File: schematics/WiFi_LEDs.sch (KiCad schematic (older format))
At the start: 8 parts

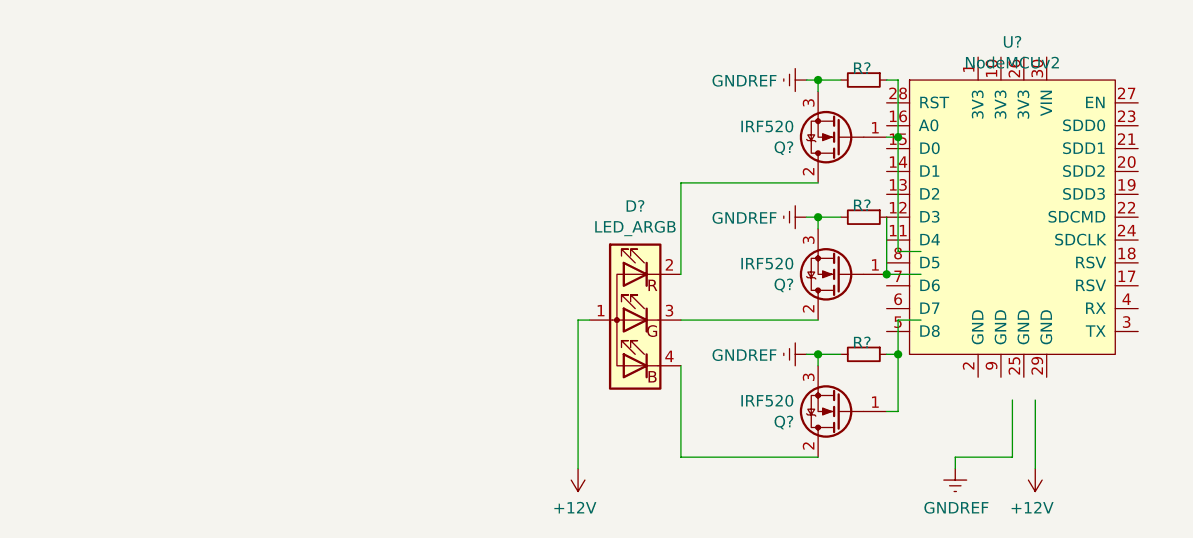
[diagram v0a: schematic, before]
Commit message: Update schematic
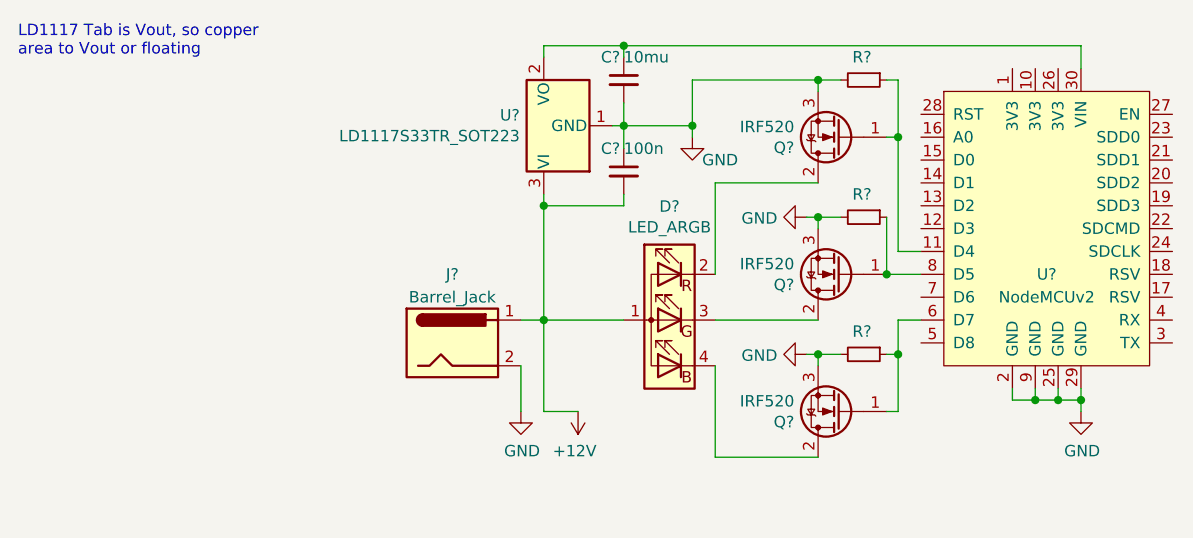
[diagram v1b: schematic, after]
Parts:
- removed U?: NodeMCUv2, symbol WiFi_LEDs:NodeMCUv2
- added C?: 10mu, symbol Device:C_Small
- added C?: 100n, symbol Device:C_Small
- added J?: Barrel_Jack, symbol Connector:Barrel_Jack
- added U?: NodeMCUv2, symbol WiFi_LEDs:NodeMCUv2
- added U?: LD1117S33TR_SOT223, Package_TO_SOT_SMD:SOT-223-3_TabPin2, symbol Regulator_Linear:LD1117S33TR_SOT223
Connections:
- net labels added: GND
- net labels removed: GNDREF
- wire segments 32 -> 54
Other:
- note added: "LD1117 Tab is Vout, so copper\narea to Vout or floating"
- moved on the sheet: D?
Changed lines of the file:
@@
 L power:+12V #PWR?
 U 1 1 60E6F443
-P 3950 3950
-F 0 "#PWR?" H 3950 3800 50  0001 C CNN
-F 1 "+12V" H 3965 4123 50  0000 C CNN
-F 2 "" H 3950 3950 50  0001 C CNN
-F 3 "" H 3950 3950 50  0001 C CNN
-	1    3950 3950
+P 3950 3700
+F 0 "#PWR?" H 3950 3550 50  0001 C CNN
+F 1 "+12V" H 3965 3873 50  0000 C CNN
+F 2 "" H 3950 3700 50  0001 C CNN
+F 3 "" H 3950 3700 50  0001 C CNN
+	1    3950 3700
 	-1   0    0    1
-$EndComp
-$Comp
-L WiFi_LEDs:NodeMCUv2 U?
-U 1 1 60E8A98C
-P 5850 2850
-F 0 "U?" H 5850 3615 50  0000 C CNN
-F 1 "NodeMCUv2" H 5850 3524 50  0000 C CNN
-F 2 "" H 5850 2050 50  0001 C CNN
-F 3 "" H 5850 2050 50  0001 C CNN
-	1    5850 2850
-	1    0    0    -1
-$EndComp
-$Comp
-L power:GNDREF #PWR?
-U 1 1 60F2CBBB
-P 4950 3450
-F 0 "#PWR?" H 4950 3200 50  0001 C CNN
-F 1 "GNDREF" V 4955 3322 50  0000 R CNN
-F 2 "" H 4950 3450 50  0001 C CNN
-F 3 "" H 4950 3450 50  0001 C CNN
-	1    4950 3450
-	0    1    1    0
-$EndComp
-$Comp
-L power:GNDREF #PWR?
-U 1 1 60F2D87A
-P 4950 2850
-F 0 "#PWR?" H 4950 2600 50  0001 C CNN
-F 1 "GNDREF" V 4955 2722 50  0000 R CNN
-F 2 "" H 4950 2850 50  0001 C CNN
-F 3 "" H 4950 2850 50  0001 C CNN
-	1    4950 2850
-	0    1    1    0
-$EndComp
-$Comp
-L power:GNDREF #PWR?
-U 1 1 60F2E231
-P 4950 2250
-F 0 "#PWR?" H 4950 2000 50  0001 C CNN
-F 1 "GNDREF" V 4955 2122 50  0000 R CNN
-F 2 "" H 4950 2250 50  0001 C CNN
-F 3 "" H 4950 2250 50  0001 C CNN
-	1    4950 2250
-	0    1    1    0
 $EndComp
 Wire Wire Line
@@
 $EndComp
 Wire Wire Line
-	4950 2250 5000 2250
-Wire Wire Line
 	5000 2250 5000 2300
 Wire Wire Line
-	3950 3950 3950 3300
-Wire Wire Line
-	3950 3300 4000 3300
-Wire Wire Line
-	4400 3100 4400 2700
-Wire Wire Line
-	4400 3500 4400 3900
-Wire Wire Line
-	4400 3900 5000 3900
-Wire Wire Line
-	4400 3300 5000 3300
+	3800 3300 4150 3300
+Wire Wire Line
+	4550 3100 4550 2700
+Wire Wire Line
+	4550 3500 4550 3900
+Wire Wire Line
+	4550 3900 5000 3900
+Wire Wire Line
+	4550 3300 5000 3300
 $Comp
 L Device:LED_ARGB D?
 U 1 1 61009E65
-P 4200 3300
-F 0 "D?" H 4200 3797 50  0000 C CNN
-F 1 "LED_ARGB" H 4200 3706 50  0000 C CNN
-F 2 "" H 4200 3250 50  0001 C CNN
-F 3 "~" H 4200 3250 50  0001 C CNN
-	1    4200 3300
+P 4350 3300
+F 0 "D?" H 4350 3797 50  0000 C CNN
+F 1 "LED_ARGB" H 4350 3706 50  0000 C CNN
+F 2 "" H 4350 3250 50  0001 C CNN
+F 3 "~" H 4350 3250 50  0001 C CNN
+	1    4350 3300
 	-1   0    0    -1
 $EndComp
 Wire Wire Line
-	4400 2700 5000 2700
+	4550 2700 5000 2700
 Wire Wire Line
 	5300 3100 5450 3100
-$Comp
-L power:+12V #PWR?
-U 1 1 61057791
-P 5950 3950
-F 0 "#PWR?" H 5950 3800 50  0001 C CNN
-F 1 "+12V" H 5965 4123 50  0000 C CNN
-F 2 "" H 5950 3950 50  0001 C CNN
-F 3 "" H 5950 3950 50  0001 C CNN
-	1    5950 3950
-	-1   0    0    1
-$EndComp
-Wire Wire Line
-	5950 3950 5950 3650
-Wire Wire Line
-	5850 3650 5850 3900
-$Comp
-L power:GNDREF #PWR?
-U 1 1 60E6DFF5
-P 5600 3950
-F 0 "#PWR?" H 5600 3700 50  0001 C CNN
-F 1 "GNDREF" H 5605 3777 50  0000 C CNN
-F 2 "" H 5600 3950 50  0001 C CNN
-F 3 "" H 5600 3950 50  0001 C CNN
-	1    5600 3950
-	1    0    0    -1
-$EndComp
-Wire Wire Line
-	5850 3900 5600 3900
-Wire Wire Line
-	5600 3900 5600 3950
 Wire Wire Line
 	5450 3300 5350 3300
@@
 U 1 1 61097AD3
 P 5200 3450
-F 0 "R?" V 5150 3400 50  0000 L CNN
+F 0 "R?" V 5100 3400 50  0000 L CNN
 F 1 "PULLDOWN" V 5150 3200 50  0001 L CNN
 F 2 "" H 5200 3450 50  0001 C CNN
@@
 U 1 1 6109ED31
 P 5200 2850
-F 0 "R?" V 5150 2800 50  0000 L CNN
+F 0 "R?" V 5100 2800 50  0000 L CNN
 F 1 "PULLDOWN" V 5150 2600 50  0001 L CNN
 F 2 "" H 5200 2850 50  0001 C CNN
@@
 U 1 1 610A4161
 P 5200 2250
-F 0 "R?" V 5150 2200 50  0000 L CNN
+F 0 "R?" V 5100 2200 50  0000 L CNN
 F 1 "PULLDOWN" V 5150 2000 50  0001 L CNN
 F 2 "" H 5200 2250 50  0001 C CNN
@@
 Wire Wire Line
 	5100 2250 5000 2250
+Wire Wire Line
+	6150 3600 6150 3650
+$Comp
+L WiFi_LEDs:NodeMCUv2 U?
+U 1 1 60EA9EFB
+P 6000 2900
+F 0 "U?" H 6000 2700 50  0000 C CNN
+F 1 "NodeMCUv2" H 6000 2600 50  0000 C CNN
+F 2 "" H 5850 1950 50  0001 C CNN
+F 3 "" H 5850 1950 50  0001 C CNN
+	1    6000 2900
+	1    0    0    -1
+$EndComp
+$Comp
+L power:GND #PWR?
+U 1 1 60EB2A98
+P 4950 2850
+F 0 "#PWR?" H 4950 2600 50  0001 C CNN
+F 1 "GND" V 4955 2722 50  0000 R CNN
+F 2 "" H 4950 2850 50  0001 C CNN
+F 3 "" H 4950 2850 50  0001 C CNN
+	1    4950 2850
+	0    1    1    0
+$EndComp
+$Comp
+L power:GND #PWR?
+U 1 1 60EB2FC7
+P 4950 3450
+F 0 "#PWR?" H 4950 3200 50  0001 C CNN
+F 1 "GND" V 4955 3322 50  0000 R CNN
+F 2 "" H 4950 3450 50  0001 C CNN
+F 3 "" H 4950 3450 50  0001 C CNN
+	1    4950 3450
+	0    1    1    0
+$EndComp
+$Comp
+L Connector:Barrel_Jack J?
+U 1 1 60EC6BDF
+P 3400 3400
+F 0 "J?" H 3400 3700 50  0000 C CNN
+F 1 "Barrel_Jack" H 3400 3600 50  0000 C CNN
+F 2 "" H 3450 3360 50  0001 C CNN
+F 3 "~" H 3450 3360 50  0001 C CNN
+	1    3400 3400
+	1    0    0    -1
+$EndComp
+Wire Wire Line
+	3700 3300 3800 3300
+$Comp
+L power:GND #PWR?
+U 1 1 60ECA6D3
+P 3700 3700
+F 0 "#PWR?" H 3700 3450 50  0001 C CNN
+F 1 "GND" H 3705 3527 50  0000 C CNN
+F 2 "" H 3700 3700 50  0001 C CNN
+F 3 "" H 3700 3700 50  0001 C CNN
+	1    3700 3700
+	1    0    0    -1
+$EndComp
+Wire Wire Line
+	3700 3500 3700 3700
+Connection ~ 3800 3300
+$Comp
+L Regulator_Linear:LD1117S33TR_SOT223 U?
+U 1 1 60ED508A
+P 3800 2450
+F 0 "U?" V 3846 2555 50  0000 L CNN
+F 1 "LD1117S33TR_SOT223" V 3755 2555 50  0000 L CNN
+F 2 "Package_TO_SOT_SMD:SOT-223-3_TabPin2" H 3800 2650 50  0001 C CNN
+F 3 "http://www.st.com/st-web-ui/static/active/en/resource/technical/document/datasheet/CD00000544.pdf" H 3900 2200 50  0001 C CNN
+	1    3800 2450
+	0    -1   -1   0
+$EndComp
+Wire Wire Line
+	3800 2750 3800 2800
+Wire Wire Line
+	3800 2150 3800 2100
+Wire Wire Line
+	3800 2100 4150 2100
+Wire Wire Line
+	6150 2100 6150 2200
+$Comp
+L power:GND #PWR?
+U 1 1 60EE74C2
+P 4450 2500
+F 0 "#PWR?" H 4450 2250 50  0001 C CNN
+F 1 "GND" H 4650 2400 50  0000 R CNN
+F 2 "" H 4450 2500 50  0001 C CNN
+F 3 "" H 4450 2500 50  0001 C CNN
+	1    4450 2500
+	1    0    0    -1
+$EndComp
+Wire Wire Line
+	5850 3600 5850 3650
+Wire Wire Line
+	5850 3650 5950 3650
+Wire Wire Line
+	5950 3600 5950 3650
+Connection ~ 5950 3650
+Wire Wire Line
+	6050 3600 6050 3650
+Connection ~ 6050 3650
+Wire Wire Line
+	6050 3650 6150 3650
+Wire Wire Line
+	5950 3650 6050 3650
+Connection ~ 6150 3650
+Wire Wire Line
+	6150 3650 6150 3700
+$Comp
+L power:GND #PWR?
+U 1 1 60EB09D8
+P 6150 3700
+F 0 "#PWR?" H 6150 3450 50  0001 C CNN
+F 1 "GND" H 6155 3527 50  0000 C CNN
+F 2 "" H 6150 3700 50  0001 C CNN
+F 3 "" H 6150 3700 50  0001 C CNN
+	1    6150 3700
+	1    0    0    -1
+$EndComp
+Wire Wire Line
+	5000 2250 4450 2250
 Connection ~ 5000 2250
+Wire Wire Line
+	4450 2250 4450 2450
+Wire Wire Line
+	4100 2450 4150 2450
+Connection ~ 4450 2450
+Wire Wire Line
+	4450 2450 4450 2500
+Wire Wire Line
+	3800 3300 3800 3700
+Wire Wire Line
+	3800 3700 3950 3700
+$Comp
+L Device:C_Small C?
+U 1 1 60F0098A
+P 4150 2250
+F 0 "C?" H 4050 2350 50  0000 L CNN
+F 1 "10mu" H 4150 2350 50  0000 L CNN
+F 2 "" H 4150 2250 50  0001 C CNN
+F 3 "~" H 4150 2250 50  0001 C CNN
+	1    4150 2250
+	1    0    0    -1
+$EndComp
+$Comp
+L Device:C_Small C?
+U 1 1 60F01DCD
+P 4150 2650
+F 0 "C?" H 4050 2750 50  0000 L CNN
+F 1 "100n" H 4150 2750 50  0000 L CNN
+F 2 "" H 4150 2650 50  0001 C CNN
+F 3 "~" H 4150 2650 50  0001 C CNN
+	1    4150 2650
+	1    0    0    -1
+$EndComp
+Wire Wire Line
+	4150 2750 4150 2800
+Wire Wire Line
+	4150 2800 3800 2800
+Connection ~ 3800 2800
+Wire Wire Line
+	3800 2800 3800 3300
+Wire Wire Line
+	4150 2550 4150 2450
+Connection ~ 4150 2450
+Wire Wire Line
+	4150 2450 4450 2450
+Wire Wire Line
+	4150 2450 4150 2350
+Wire Wire Line
+	4150 2150 4150 2100
+Connection ~ 4150 2100
+Wire Wire Line
+	4150 2100 6150 2100
+Text Notes 1500 2150 0    50   ~ 0
+LD1117 Tab is Vout, so copper\narea to Vout or floating
 $EndSCHEMATC
